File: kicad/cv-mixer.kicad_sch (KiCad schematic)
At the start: 19 parts, among them J21 Eurorack Mono Jack, J22 Eurorack Mono Jack, J23 Eurorack Mono Jack, J48 Eurorack Mono Jack, U21 TL072

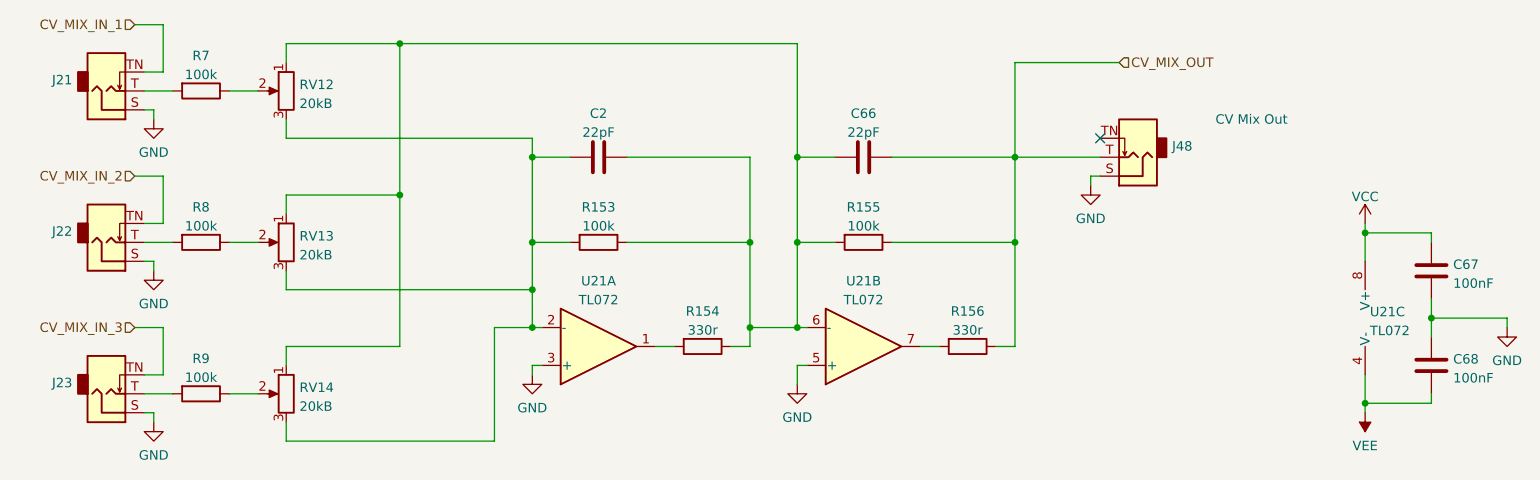
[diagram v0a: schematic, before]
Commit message: Final changes for rev01
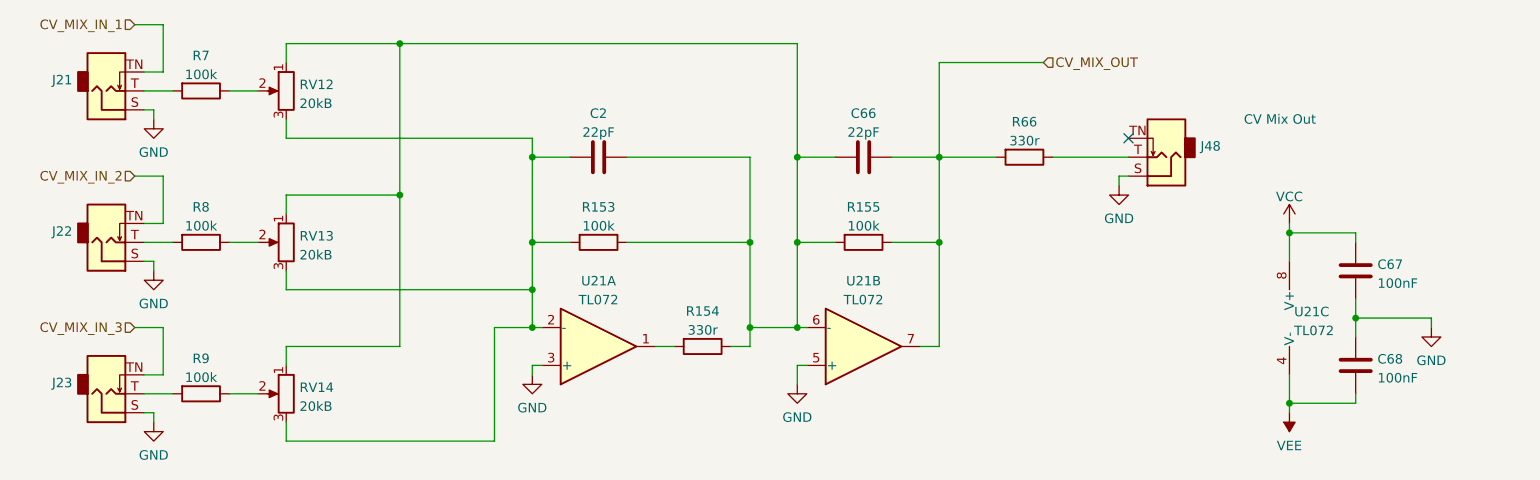
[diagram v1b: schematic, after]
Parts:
- removed R156: 330r, rumblesan-standard-parts:R_Axial_DIN0207_L6.3mm_D2.5mm_P10.16mm_Horizontal, symbol rumblesan-standard-parts:R
- added R66: 330r, rumblesan-standard-parts:R_Axial_DIN0207_L6.3mm_D2.5mm_P10.16mm_Horizontal, symbol rumblesan-standard-parts:R
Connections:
- net CV_MIX_OUT: now also U21.7, R66.2; no longer J48.T (Tip)
- new net: J48.T (Tip), R66.1
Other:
- moved on the sheet: C67, C68, J48, U21C
